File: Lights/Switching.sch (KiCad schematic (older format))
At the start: 7 parts, among them J401 Light, Q401 PN2222A, Q402 IRF540N, U401 6N138

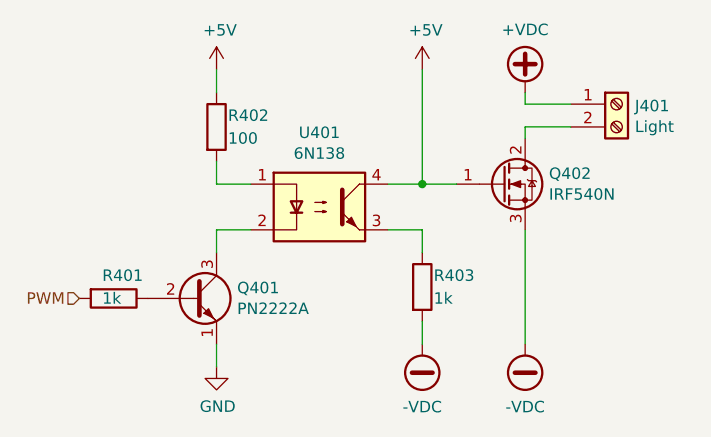
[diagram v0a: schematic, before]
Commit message: Finished schematic and routing
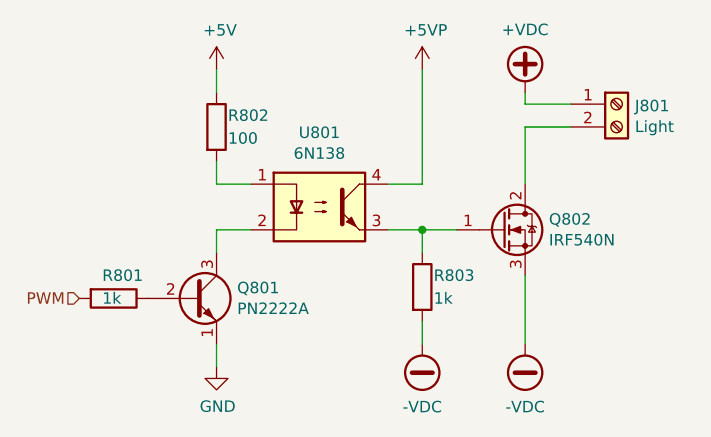
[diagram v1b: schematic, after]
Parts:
- R401, R402, R403: footprint Resistor_THT:R_Axial_DIN0204_L3.6mm_D1.6mm_P7.62mm_Horizontal -> Resistor_THT:R_Axial_DIN0204_L3.6mm_D1.6mm_P2.54mm_Vertical
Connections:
- net +5V: no longer Q402.1 (G), U401.4
- net at R403.1, U401.3: now also Q402.1 (G)
- new net +5VP: U401.4
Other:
- moved on the sheet: Q802
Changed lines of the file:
@@
 $Descr A4 11693 8268
 encoding utf-8
-Sheet 4 8
+Sheet 8 8
 Title ""
 Date ""
@@
 AR Path="/60725945/60687108" Ref="U701"  Part="1"
 AR Path="/607266E0/60687108" Ref="U801"  Part="1"
-F 0 "U401" H 1900 1775 50  0000 C CNN
+F 0 "U801" H 1900 1775 50  0000 C CNN
 F 1 "6N138" H 1900 1684 50  0000 C CNN
 F 2 "Package_DIP:DIP-4_W7.62mm" H 1700 1250 50  0001 L CIN
@@
 AR Path="/60725945/60689BC6" Ref="R702"  Part="1"
 AR Path="/607266E0/60689BC6" Ref="R802"  Part="1"
-F 0 "R402" H 1500 1150 50  0000 L CNN
+F 0 "R802" H 1500 1150 50  0000 L CNN
 F 1 "100" H 1500 1050 50  0000 L CNN
-F 2 "Resistor_THT:R_Axial_DIN0204_L3.6mm_D1.6mm_P7.62mm_Horizontal" V 1380 1100 50  0001 C CNN
+F 2 "Resistor_THT:R_Axial_DIN0204_L3.6mm_D1.6mm_P2.54mm_Vertical" V 1380 1100 50  0001 C CNN
 F 3 "~" H 1450 1100 50  0001 C CNN
 	1    1450 1100
@@
 AR Path="/60725945/6068FB2D" Ref="Q701"  Part="1"
 AR Path="/607266E0/6068FB2D" Ref="Q801"  Part="1"
-F 0 "Q401" H 1540 1896 50  0000 L CNN
+F 0 "Q801" H 1540 1896 50  0000 L CNN
 F 1 "PN2222A" H 1540 1805 50  0000 L CNN
 F 2 "Package_TO_SOT_THT:TO-92_Inline_Wide" H 1550 1775 50  0001 L CIN
@@
 AR Path="/60725945/60692608" Ref="R701"  Part="1"
 AR Path="/607266E0/60692608" Ref="R801"  Part="1"
-F 0 "R401" V 900 1800 50  0000 L CNN
+F 0 "R801" V 900 1800 50  0000 L CNN
 F 1 "1k" V 1000 1800 50  0000 L CNN
-F 2 "Resistor_THT:R_Axial_DIN0204_L3.6mm_D1.6mm_P7.62mm_Horizontal" V 930 1850 50  0001 C CNN
+F 2 "Resistor_THT:R_Axial_DIN0204_L3.6mm_D1.6mm_P2.54mm_Vertical" V 930 1850 50  0001 C CNN
 F 3 "~" H 1000 1850 50  0001 C CNN
 	1    1000 1850
@@
 AR Path="/60725945/60698CBE" Ref="#PWR0701"  Part="1"
 AR Path="/607266E0/60698CBE" Ref="#PWR0801"  Part="1"
-F 0 "#PWR0401" H 1450 700 50  0001 C CNN
+F 0 "#PWR0801" H 1450 700 50  0001 C CNN
 F 1 "+5V" H 1465 1023 50  0000 C CNN
 F 2 "" H 1450 850 50  0001 C CNN
@@
 AR Path="/60725945/6069909C" Ref="#PWR0702"  Part="1"
 AR Path="/607266E0/6069909C" Ref="#PWR0802"  Part="1"
-F 0 "#PWR0402" H 1450 1900 50  0001 C CNN
+F 0 "#PWR0802" H 1450 1900 50  0001 C CNN
 F 1 "GND" H 1455 1977 50  0000 C CNN
 F 2 "" H 1450 2150 50  0001 C CNN
@@
 AR Path="/60725945/6069AD31" Ref="R703"  Part="1"
 AR Path="/607266E0/6069AD31" Ref="R803"  Part="1"
-F 0 "R403" H 2400 1850 50  0000 L CNN
+F 0 "R803" H 2400 1850 50  0000 L CNN
 F 1 "1k" H 2400 1750 50  0000 L CNN
-F 2 "Resistor_THT:R_Axial_DIN0204_L3.6mm_D1.6mm_P7.62mm_Horizontal" V 2280 1800 50  0001 C CNN
+F 2 "Resistor_THT:R_Axial_DIN0204_L3.6mm_D1.6mm_P2.54mm_Vertical" V 2280 1800 50  0001 C CNN
 F 3 "~" H 2350 1800 50  0001 C CNN
 	1    2350 1800
 	1    0    0    -1
 $EndComp
-$Comp
-L power:+5V #PWR0403
-U 1 1 6069AD39
-P 2350 850
-AR Path="/60632B44/6069AD39" Ref="#PWR0403"  Part="1"
-AR Path="/60725945/6069AD39" Ref="#PWR0703"  Part="1"
-AR Path="/607266E0/6069AD39" Ref="#PWR0803"  Part="1"
-F 0 "#PWR0403" H 2350 700 50  0001 C CNN
-F 1 "+5V" H 2365 1023 50  0000 C CNN
-F 2 "" H 2350 850 50  0001 C CNN
-F 3 "" H 2350 850 50  0001 C CNN
-	1    2350 850
-	1    0    0    -1
-$EndComp
 Wire Wire Line
 	2350 1950 2350 2050
@@
 L Transistor_FET:IRF540N Q402
 U 1 1 6069E315
-P 2700 1350
+P 2700 1550
 AR Path="/60632B44/6069E315" Ref="Q402"  Part="1"
 AR Path="/60725945/6069E315" Ref="Q702"  Part="1"
 AR Path="/607266E0/6069E315" Ref="Q802"  Part="1"
-F 0 "Q402" H 2904 1396 50  0000 L CNN
-F 1 "IRF540N" H 2904 1305 50  0000 L CNN
-F 2 "Package_TO_SOT_THT:TO-220-3_Vertical" H 2950 1275 50  0001 L CIN
-F 3 "http://www.irf.com/product-info/datasheets/data/irf540n.pdf" H 2700 1350 50  0001 L CNN
-	1    2700 1350
-	1    0    0    -1
-$EndComp
-Wire Wire Line
-	2800 1550 2800 2050
-Wire Wire Line
-	2500 1350 2350 1350
-Connection ~ 2350 1350
+F 0 "Q802" H 2904 1596 50  0000 L CNN
+F 1 "IRF540N" H 2904 1505 50  0000 L CNN
+F 2 "Package_TO_SOT_THT:TO-220-3_Vertical" H 2950 1475 50  0001 L CIN
+F 3 "http://www.irf.com/product-info/datasheets/data/irf540n.pdf" H 2700 1550 50  0001 L CNN
+	1    2700 1550
+	1    0    0    -1
+$EndComp
+Wire Wire Line
+	2800 1750 2800 2050
 Wire Wire Line
 	2200 1350 2350 1350
@@
 AR Path="/60725945/606AE8B7" Ref="#PWR0704"  Part="1"
 AR Path="/607266E0/606AE8B7" Ref="#PWR0804"  Part="1"
-F 0 "#PWR0404" H 2350 1950 50  0001 C CNN
+F 0 "#PWR0804" H 2350 1950 50  0001 C CNN
 F 1 "-VDC" H 2350 2325 50  0000 C CNN
 F 2 "" H 2350 2050 50  0001 C CNN
@@
 AR Path="/60725945/606AF7CF" Ref="#PWR0706"  Part="1"
 AR Path="/607266E0/606AF7CF" Ref="#PWR0806"  Part="1"
-F 0 "#PWR0406" H 2800 1950 50  0001 C CNN
+F 0 "#PWR0806" H 2800 1950 50  0001 C CNN
 F 1 "-VDC" H 2800 2325 50  0000 C CNN
 F 2 "" H 2800 2050 50  0001 C CNN
@@
 AR Path="/60725945/606AFF23" Ref="#PWR0705"  Part="1"
 AR Path="/607266E0/606AFF23" Ref="#PWR0805"  Part="1"
-F 0 "#PWR0405" H 2800 850 50  0001 C CNN
+F 0 "#PWR0805" H 2800 850 50  0001 C CNN
 F 1 "+VDC" H 2800 1225 50  0000 C CNN
 F 2 "" H 2800 950 50  0001 C CNN
@@
 AR Path="/60725945/606B0F32" Ref="J701"  Part="1"
 AR Path="/607266E0/606B0F32" Ref="J801"  Part="1"
-F 0 "J401" H 3280 992 50  0000 L CNN
+F 0 "J801" H 3280 992 50  0000 L CNN
 F 1 "Light" H 3280 901 50  0000 L CNN
 F 2 "TerminalBlock:TerminalBlock_bornier-2_P5.08mm" H 3200 1000 50  0001 C CNN
@@
 	3000 1100 2800 1100
 Wire Wire Line
-	2800 1100 2800 1150
+	2800 1100 2800 1350
+Wire Wire Line
+	2500 1550 2350 1550
+Connection ~ 2350 1550
+$Comp
+L power:+5VP #PWR?
+U 1 1 60B137D4
+P 2350 850
+AR Path="/60B137D4" Ref="#PWR?"  Part="1"
+AR Path="/60632B44/60B137D4" Ref="#PWR0158"  Part="1"
+AR Path="/60725945/60B137D4" Ref="#PWR0159"  Part="1"
+AR Path="/607266E0/60B137D4" Ref="#PWR0160"  Part="1"
+F 0 "#PWR0160" H 2350 700 50  0001 C CNN
+F 1 "+5VP" H 2365 1023 50  0000 C CNN
+F 2 "" H 2350 850 50  0001 C CNN
+F 3 "" H 2350 850 50  0001 C CNN
+	1    2350 850
+	1    0    0    -1
+$EndComp
 $EndSCHEMATC
